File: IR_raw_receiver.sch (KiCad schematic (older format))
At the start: 5 parts

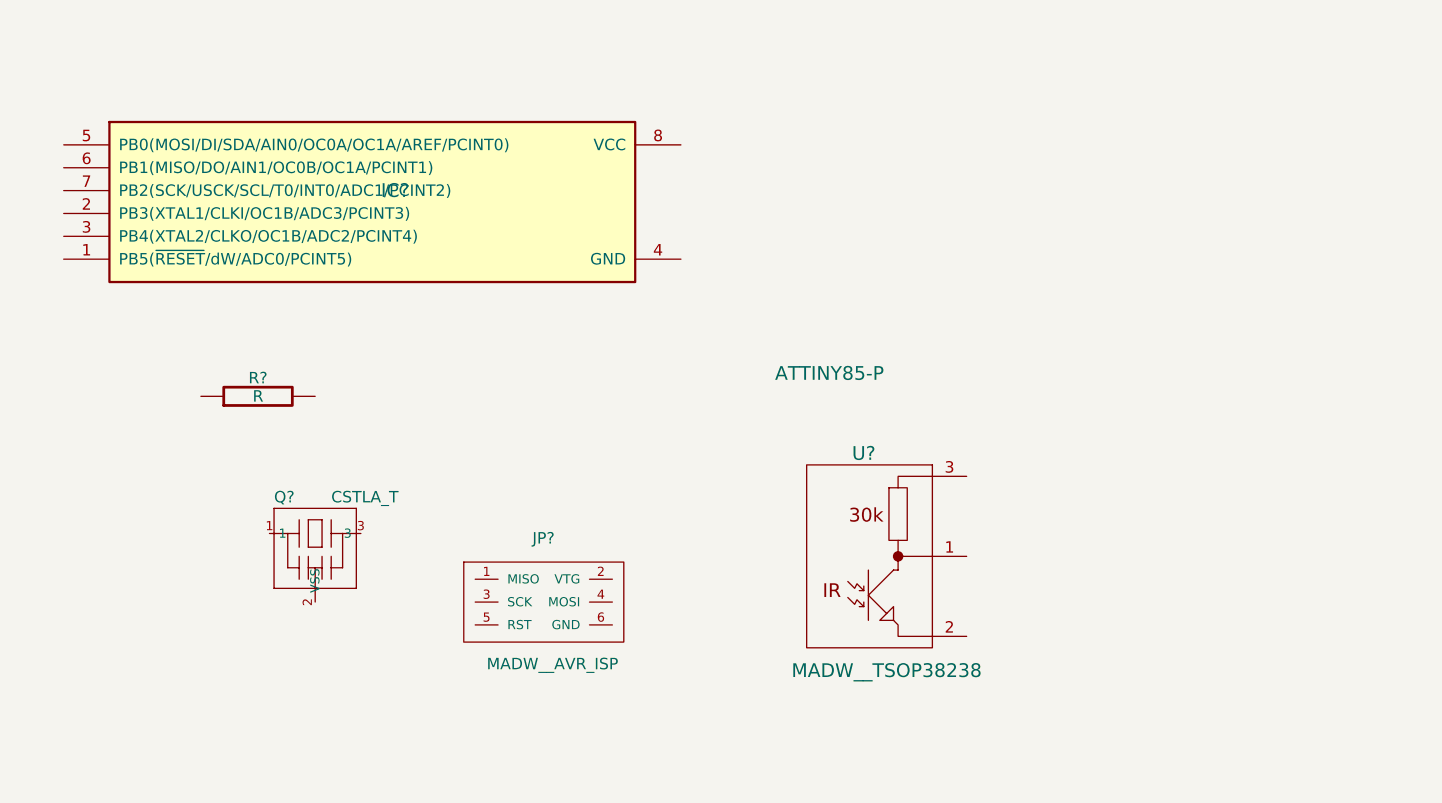
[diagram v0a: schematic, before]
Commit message: Might be done already :-)
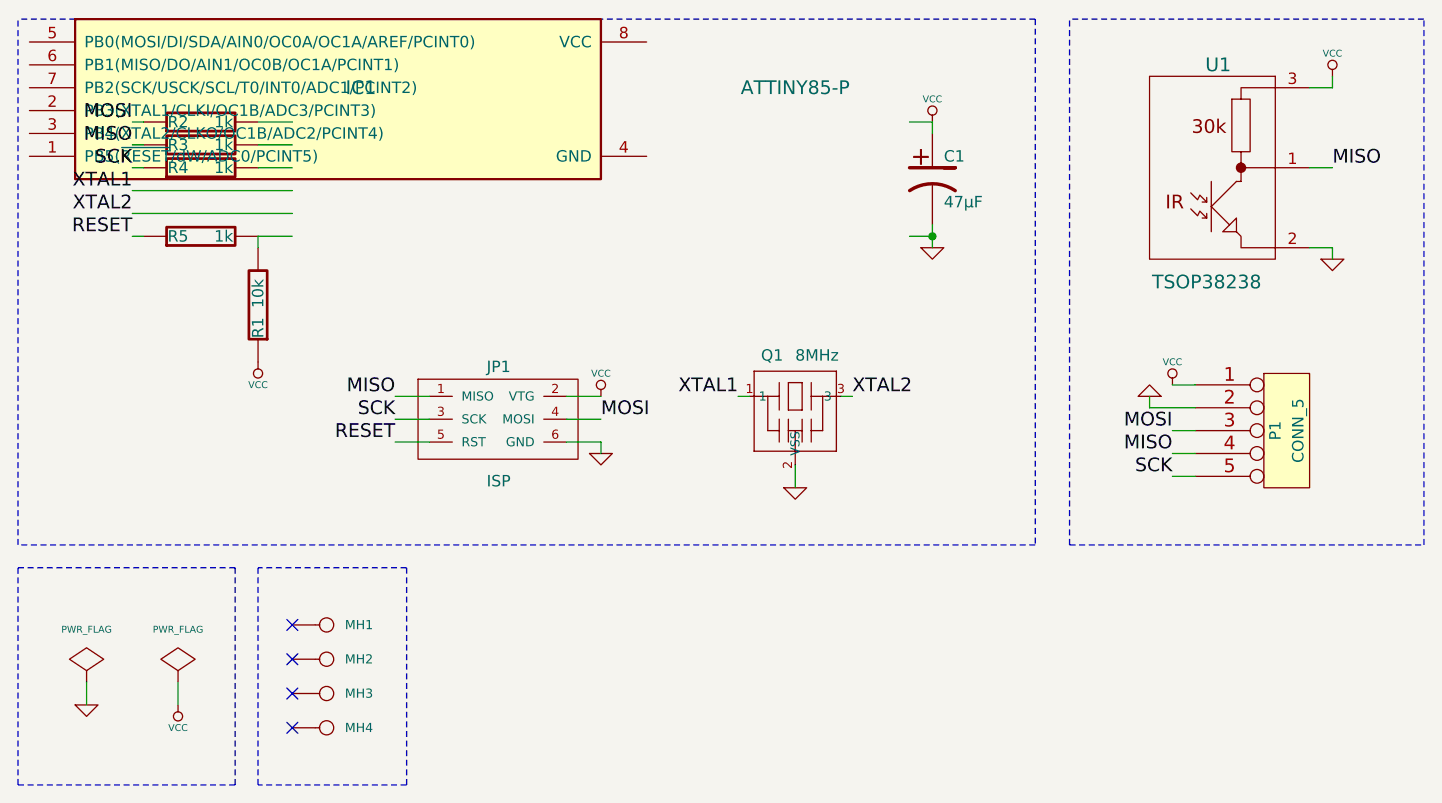
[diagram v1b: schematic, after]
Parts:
- added C1: 47µF, symbol CP1
- added MH1, MH2, MH3, MH4: CONN_1, symbol CONN_1
- added P1: CONN_5, symbol CONN_5
- added R2, R3, R4, R5: 1k, symbol R
- JP1: renamed from JP?; value MADW__AVR_ISP -> ISP
- Q1: renamed from Q?; value CSTLA_T -> 8MHz
- R1: renamed from R?; value R -> 10k
- U1: renamed from U?; value MADW__TSOP38238 -> TSOP38238
- gave numbers to parts that had none: 1
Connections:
- net labels added: GND, MISO, MOSI, RESET, SCK, VCC, XTAL1, XTAL2
- wire segments 0 -> 38
- no-connect marks 0 -> 4
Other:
- moved on the sheet: IC1, JP1, Q1, R1, U1
